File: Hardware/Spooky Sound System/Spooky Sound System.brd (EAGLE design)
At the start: 101.6 x 77.2 mm, 85 parts, among them J1 SJ1-3533NS, J2 1546215-2, J3 1546215-2, J4 1546215-2, J5 1546215-2, U1 TDA7387, U2 AZ4558C, U3 AZ4558C, U4 AZ4558C, U5 AZ4558C, U6 AZ4558C

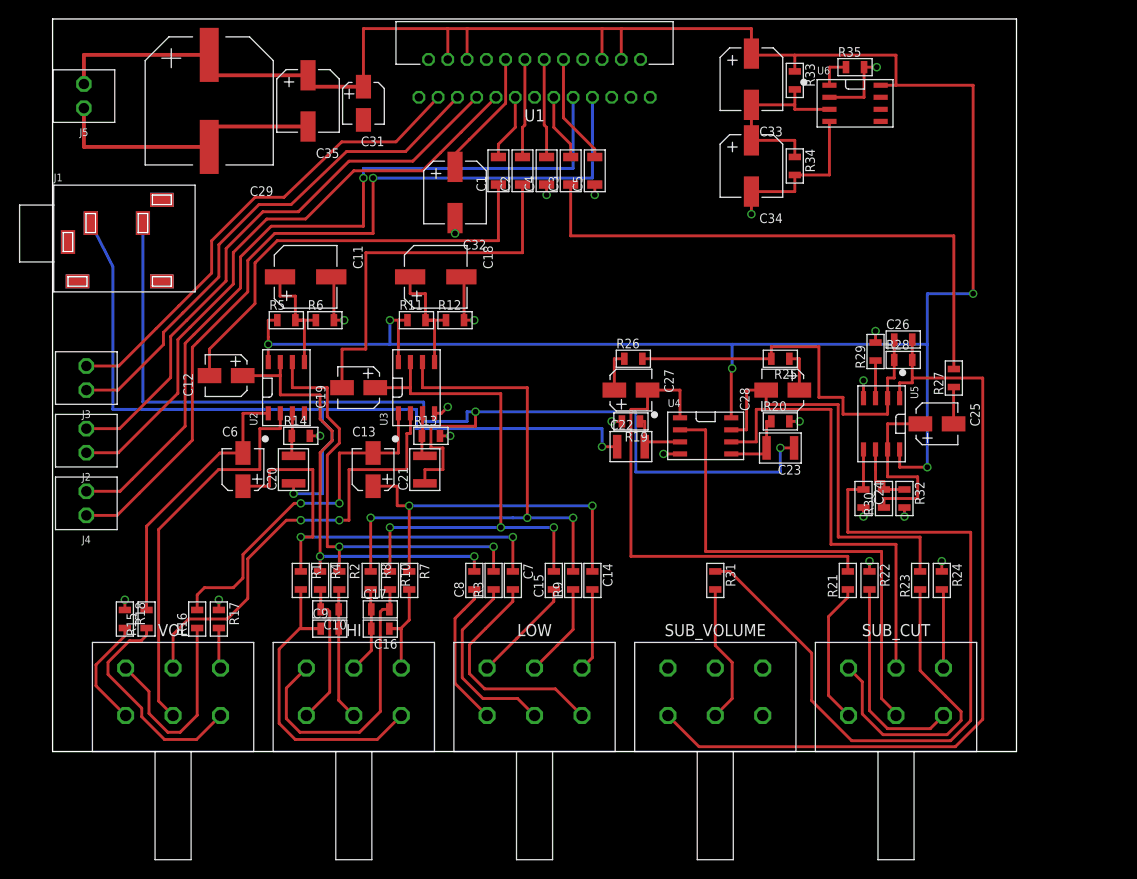
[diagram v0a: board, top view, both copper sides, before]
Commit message: Finished routing
Just needs tweaking and final look over.
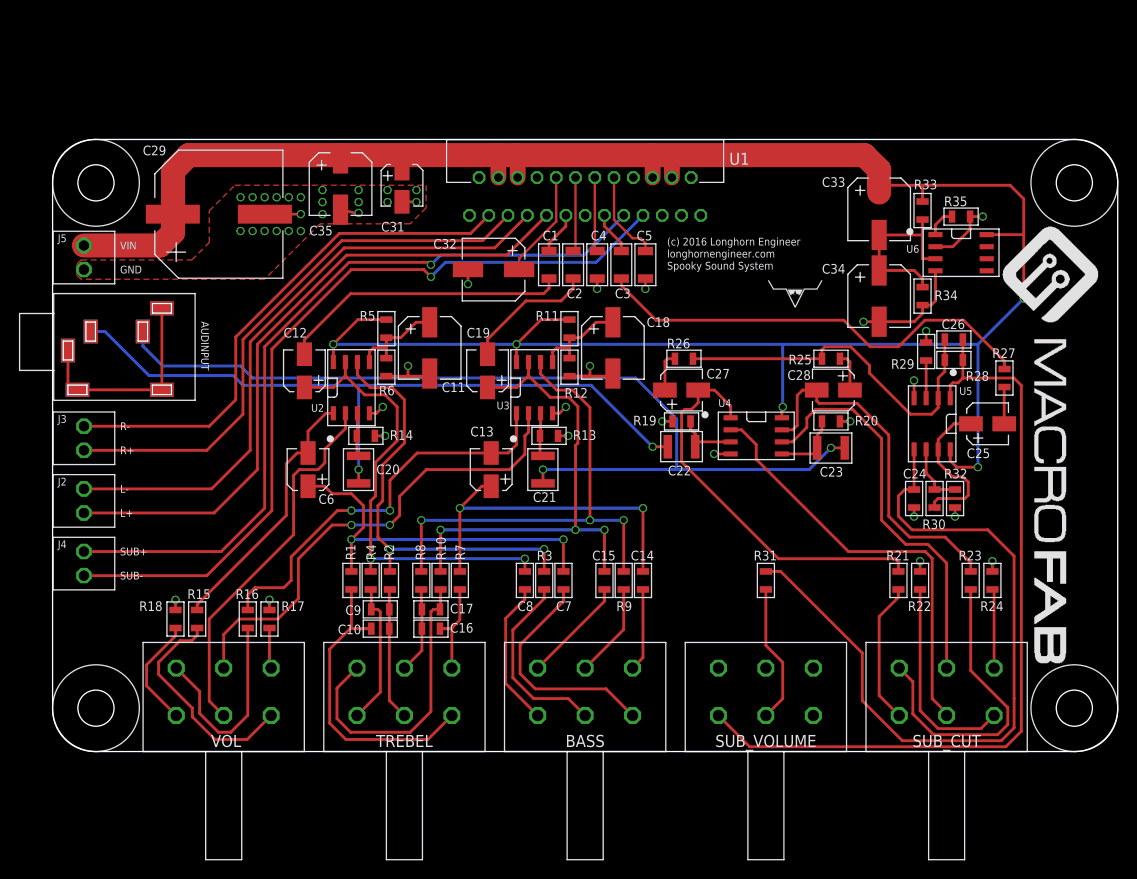
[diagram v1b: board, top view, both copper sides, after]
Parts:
- removed HI, LOW: 100K, PP_Passives:DUAL_TAPER_POTENTIOMETER
- removed J1: SJ1-3533NS, PP_Connectors:SJ1-3533NS
- added AUDINPUT: SJ1-3533NS, PP_Connectors:SJ1-3533NS
- added BASS, TREBEL: 100K, PP_Passives:DUAL_TAPER_POTENTIOMETER
- added H1, H2, H3, H4: MOUNT_HOLE150MIL, PP_Connectors:MOUNT_HOLE_150MIL
- added LOGO1: SPOOKY_LOGOSPOOKY_LOGO, PP_Aesthetics:SPOOKY_LOGO
- added U$17: LHE_FRAME, PP_Aesthetics:LHE_FRAME
- added U$18: LHE_LOGOLHE_LOGO, PP_Aesthetics:LHE_LOGO
- added U$19: MF_LOGOLOGO_TEXT, PP_Aesthetics:MF_LOGO_TEXT
- moved C18 20.1 mm to (59.1, 42.5), turned to 180 degrees
- moved R35 19.3 mm to (95.8, 56.4)
- moved U6 19.3 mm to (95.8, 52.6)
- moved C33 19.2 mm to (87.1, 57.1)
- moved C34 19.2 mm to (87.1, 48.0)
- moved R33 19.2 mm to (91.7, 57.0)
- moved R34 19.2 mm to (91.7, 48.0)
- moved J5 17.0 mm to (3.30, 52.1)
- moved R11 16.2 mm to (54.5, 44.6), turned to 270 degrees
- moved C11 15.1 mm to (39.8, 42.5), turned to 180 degrees
- moved C19 13.7 mm to (45.8, 40.1), turned to 0 degrees
- moved U1 13.5 mm to (56.1, 56.5)
- moved R12 13.0 mm to (54.5, 40.5), turned to 270 degrees
- moved C13 12.4 mm to (46.2, 29.7)
- moved C21 12.4 mm to (51.7, 29.7)
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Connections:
- net AUD_IN_L: now also AUDINPUT.2_A, AUDINPUT.2_B; no longer J1.2_A, J1.2_B
- net AUD_IN_R: now also AUDINPUT.3_A, AUDINPUT.3_B; no longer J1.3_A, J1.3_B
- net GND: now also AUDINPUT.1_A, AUDINPUT.1_B, AUDINPUT.S1, AUDINPUT.S2, AUDINPUT.S3, AUDINPUT.S4, AUDINPUT.S5, AUDINPUT.S6; no longer J1.1_A, J1.1_B, J1.S1, J1.S2, J1.S3, J1.S4, J1.S5, J1.S6
- net N$14: now also TREBEL.1B; no longer HI.1B
- net N$15: now also TREBEL.2B; no longer HI.2B
- net N$16: now also TREBEL.3B; no longer HI.3B
- net N$18: now also BASS.2B; no longer LOW.2B
- net N$19: now also BASS.1B; no longer LOW.1B
- net N$20: now also BASS.3B; no longer LOW.3B
- net N$3: now also TREBEL.1A; no longer HI.1A
- net N$4: now also TREBEL.2A; no longer HI.2A
- net N$5: now also TREBEL.3A; no longer HI.3A
- net N$7: now also BASS.2A; no longer LOW.2A
- net N$8: now also BASS.1A; no longer LOW.1A
- net N$9: now also BASS.3A; no longer LOW.3A
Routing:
- net GND: track 59.5 -> 91.9 mm, vias 7 -> 31
- net OUT_R: track 40.4 -> 13.9 mm
- net OUT_L: track 46.4 -> 30.6 mm
- net AUD_IN_L: track 91.2 -> 76.2 mm
- net AUD_IN_R: track 114.9 -> 100.5 mm
- net OUT_SUB: track 59.8 -> 47.6 mm
- net VIN: track 269.8 -> 260.8 mm
- net N$17: track 60.1 -> 51.9 mm
- net N$23: track 50.1 -> 42.3 mm
- net N$2: track 47.1 -> 39.9 mm
- net N$35: track 52.0 -> 45.0 mm
- net N$38: track 48.1 -> 42.2 mm
- net N$27: track 43.2 -> 37.6 mm
- net L+: track 64.0 -> 69.5 mm
- net N$12: track 37.7 -> 43.1 mm
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- added copper zone on layer 1, net GND
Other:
- board size 101.6 x 77.2 mm -> 112.3 x 64.5 mm
